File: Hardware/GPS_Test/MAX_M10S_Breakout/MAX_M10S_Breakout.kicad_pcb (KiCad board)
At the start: 4 copper layers, 32.1 x 28.6 mm, 15 parts, among them J1 U.FL-R-SMT(01), J2 Conn_01x10, U1 MAX-M10S

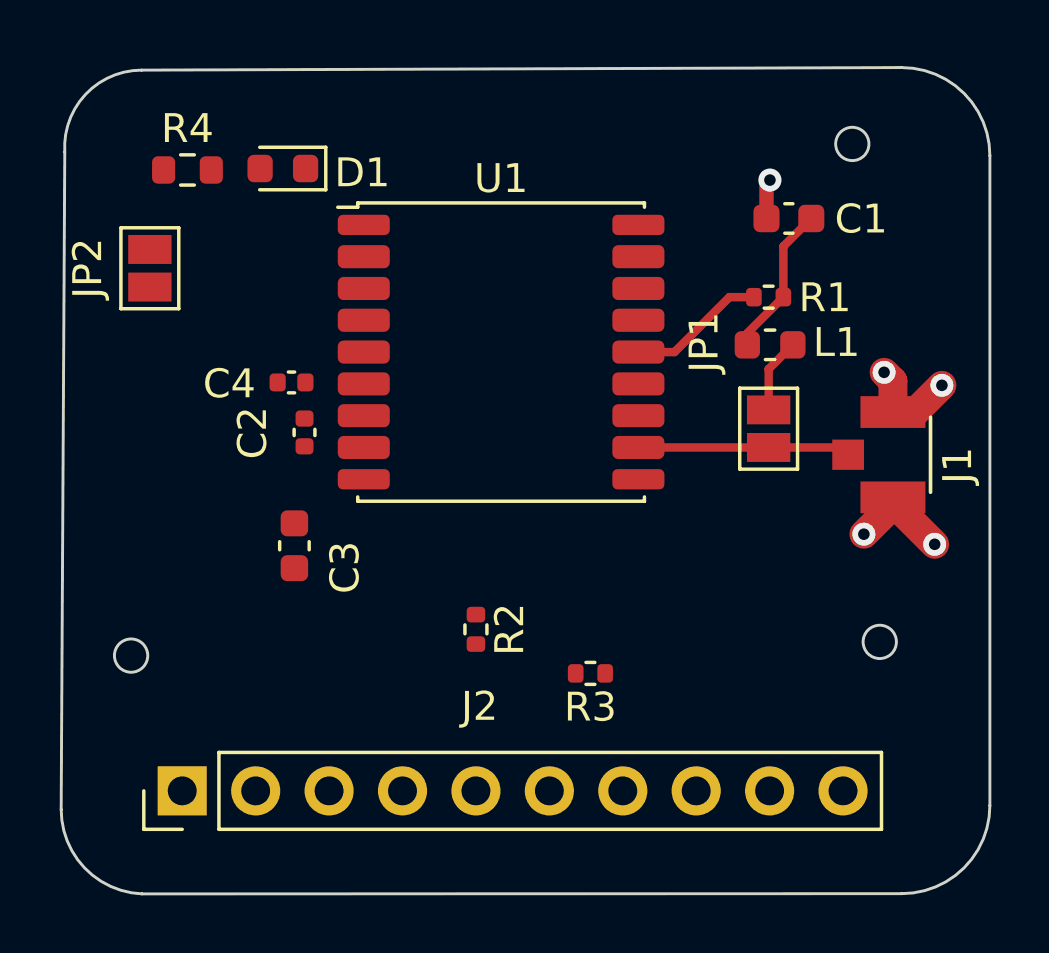
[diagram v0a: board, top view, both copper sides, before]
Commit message: Max-M10S finished
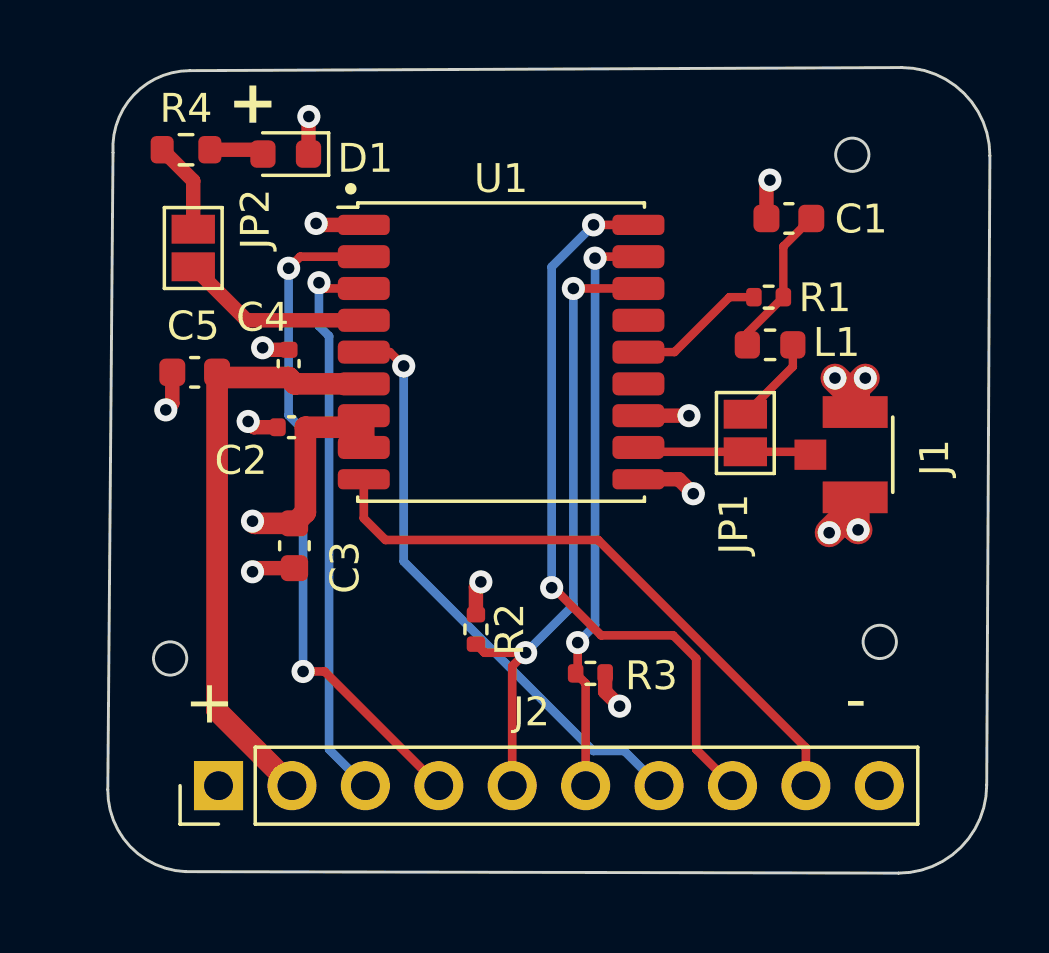
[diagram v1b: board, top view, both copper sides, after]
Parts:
- added C5: 4.7uF, Capacitor_SMD:C_0603_1608Metric, F.Cu at (84.2, 54.1)
- moved JP2 1.66 mm to (84.2, 49.8)
- moved J1 1.31 mm to (107.1, 57.0)
- moved J2 1.27 mm to (85.1, 68.4)
- moved JP1 0.82 mm to (103.3, 56.2)
- moved R4 0.70 mm to (84.0, 46.4)
- moved C4 0.66 mm to (87.5, 53.8), turned to 90 degrees
- moved D1 0.51 mm to (87.4, 46.5)
- moved C2 0.48 mm to (87.6, 56.0), turned to 180 degrees
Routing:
- net ~{SAFE}: track 0.00 -> 25.6 mm, vias 0 -> 2
- net TX: track 0.00 -> 23.3 mm, vias 0 -> 2
- net SDA: track 0.00 -> 22.2 mm, vias 0 -> 2
- net ~{RESET}: track 0.00 -> 21.2 mm
- net +BATT: track 0.00 -> 20.6 mm
- net INT: track 0.00 -> 20.4 mm, vias 0 -> 1
- net SCL: track 0.00 -> 20.2 mm, vias 0 -> 2
- net RX: track 0.00 -> 19.7 mm, vias 0 -> 1
- net +3.3V: track 0.00 -> 10.8 mm, vias 0 -> 3
- net GND: track 8.87 -> 18.7 mm, vias 5 -> 13
- net PPS: track 0.00 -> 6.67 mm
- net Net-(JP2-A): track 0.00 -> 3.20 mm
- net Net-(D1-A): track 0.00 -> 1.90 mm
- net Net-(J1-SIG): track 7.36 -> 6.05 mm
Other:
- board size 32.1 x 28.6 mm -> 30.5 x 27.9 mm
- board text added: "+"
- board text added: "-"
- board text added: "BATT"
- board text added: "INT"
- board text added: "Max-M10S Breakout Board"
- board text added: "RX"
- board text added: "SCL"
- board text added: "SDA"
- board text added: "TX"
- board text added: "~{RESET}"
- board text added: "~{SAFE}"
